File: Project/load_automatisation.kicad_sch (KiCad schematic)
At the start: 32 parts, among them IC1 TD62083AFGNEL, IC10 TD62083AFGNEL, IC2 TD62083AFGNEL, IC3 MC74VHC138DR2G, IC4 MC74VHC138DR2G, IC5 MC74VHC138DR2G, IC6 TD62083AFGNEL, IC7 TD62083AFGNEL, IC8 TD62083AFGNEL, IC9 LM358PWG4, J10 TENGConnector, J11 TENG, J12 PH-2X05SG, J19 DaqConnector, J9 PowerIn, Q1 2N5457, Q2 2N5457, U1 AMS1117-5.0, U2 INA128

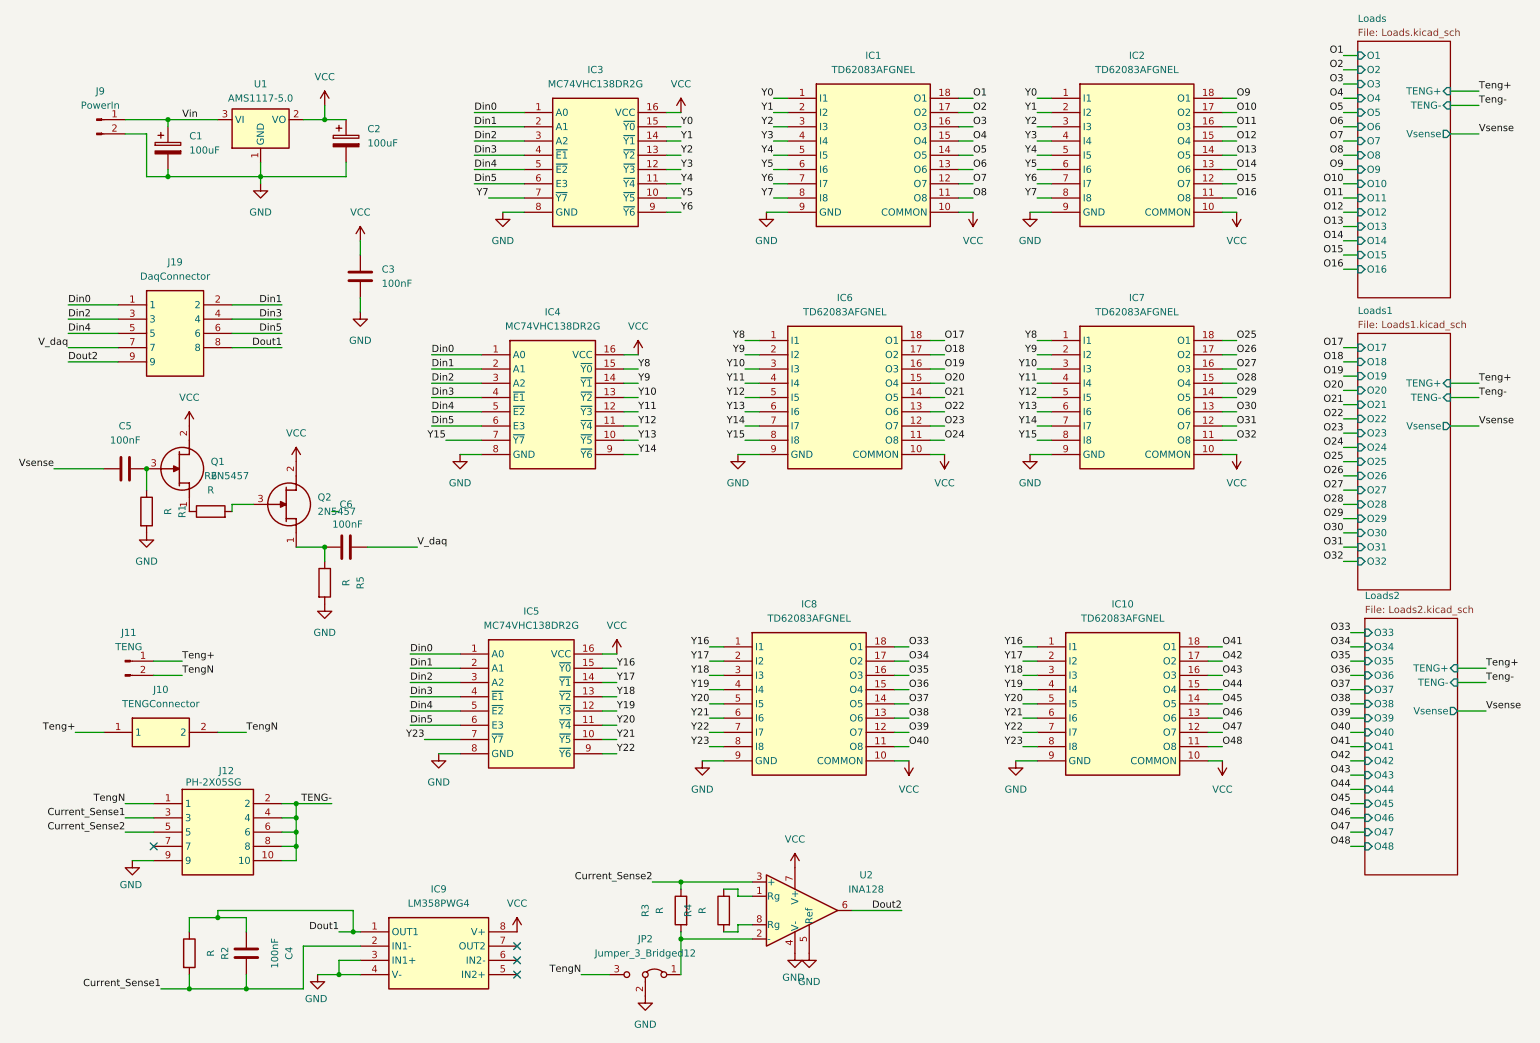
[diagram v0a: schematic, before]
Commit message: new 08/11
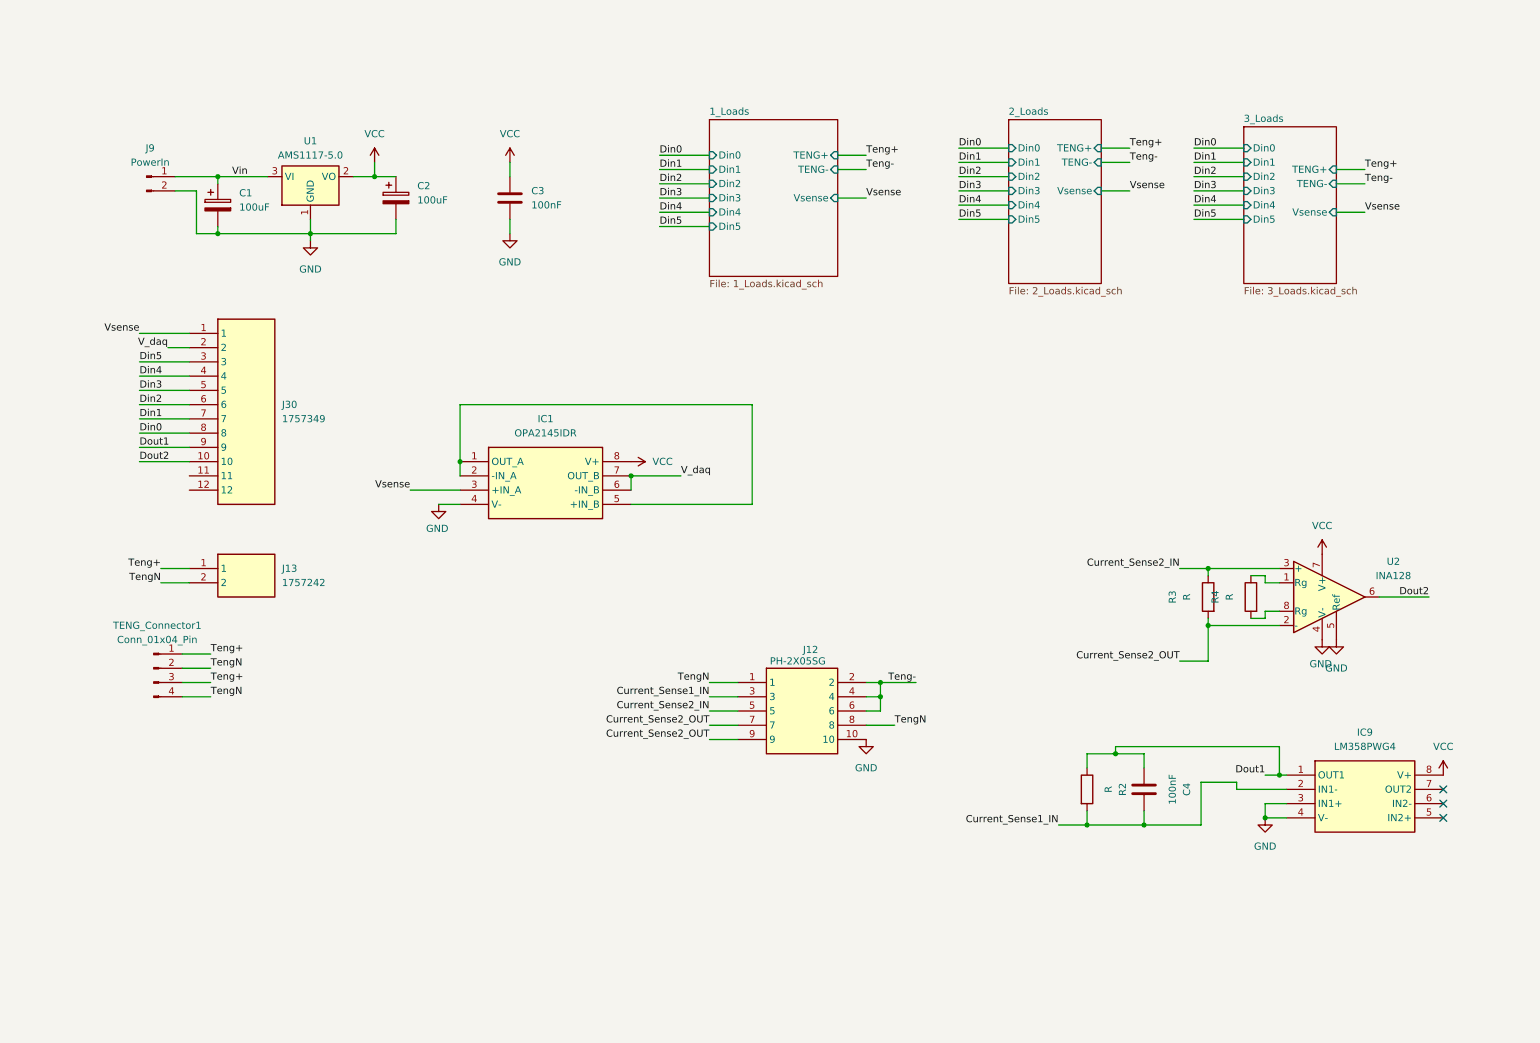
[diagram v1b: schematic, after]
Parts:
- removed C5, C6: 100nF, Capacitor_SMD:C_0805_2012Metric, symbol Device:C
- removed IC1, IC10, IC2, IC6, IC7, IC8: TD62083AFGNEL, SOIC127P1030X245-18N, symbol SamacSys_Parts:TD62083AFGNEL
- removed IC3: MC74VHC138DR2G, Library:SOIC127P600X175-16N, symbol SamacSys_Parts:MC74VHC138DR2G
- removed IC4, IC5: MC74VHC138DR2G, SamacSys_Parts:SOIC127P600X175-16N, symbol SamacSys_Parts:MC74VHC138DR2G
- removed J10: TENGConnector, 231162001000, symbol SamacSys_Parts:231-162_001-000
- removed J11: TENG, Connector_PinHeader_2.54mm:PinHeader_1x02_P2.54mm_Vertical, symbol Connector:Conn_01x02_Pin
- removed J19: DaqConnector, 231339001000, symbol SamacSys_Parts:231-339_001-000
- removed JP2: Jumper_3_Bridged12, Jumper:SolderJumper-3_P1.3mm_Bridged2Bar12_Pad1.0x1.5mm_NumberLabels, symbol Jumper:Jumper_3_Bridged12
- removed Q1, Q2: 2N5457, PN4117, symbol SamacSys_Parts:2N5457
- removed R1, R5, R6: R, Resistor_SMD:R_0805_2012Metric, symbol Device:R
- added IC1: OPA2145IDR, SOIC127P600X175-8N, symbol SamacSys_Parts:OPA2145IDR
- added J13: 1757242, 1757242, symbol SamacSys_Parts:1757242
- added J30: 1757349, SHDRRA12W103P0X508_1X12_6296X1200X875P, symbol SamacSys_Parts:1757349
- added TENG_Connector1: Conn_01x04_Pin, Connector_PinHeader_2.54mm:PinHeader_1x04_P2.54mm_Vertical, symbol Connector:Conn_01x04_Pin
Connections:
- net Din0: now also J30.8
- net Din1: now also J30.7
- net Din2: now also J30.6
- net Din3: now also J30.5
- net Din4: now also J30.4
- net Din5: now also J30.3
- net Dout1: now also J30.9
- net Dout2: now also J30.10
- net GND: now also J12.10, IC1.4 (V-); no longer J12.9
- net Teng+: now also J13.1, TENG_Connector1.1 (Pin_1), TENG_Connector1.3 (Pin_3)
- net Teng-: now also J12.2, J12.4, J12.6
- net TengN: now also J12.8, J13.2, TENG_Connector1.2 (Pin_2), TENG_Connector1.4 (Pin_4)
- net VCC: now also IC1.8 (V+)
- net V_daq: now also IC1.6 (-IN_B), IC1.7 (OUT_B), J30.2
- net Vsense: now also IC1.3 (+IN_A), J30.1
- net Current_Sense2_OUT: now reaches J12.7
- net Current_Sense2_OUT: now also J12.9, R3.2, U2.2 (-)
- net Current_Sense1 renamed Current_Sense1_IN
- net Current_Sense2 renamed Current_Sense2_IN
- removed net TENG-: J12.10, J12.2, J12.4, J12.6, J12.8
- new net: IC1.1 (OUT_A), IC1.2 (-IN_A), IC1.5 (+IN_B)
- no-connect marks 4 -> 3
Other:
- removed sheet Loads
- removed sheet Loads1
- removed sheet Loads2
- added sheet 1_Loads (1_Loads.kicad_sch)
- added sheet 2_Loads (2_Loads.kicad_sch)
- added sheet 3_Loads (3_Loads.kicad_sch)
- moved on the sheet: C1, C2, C3, C4, IC9, J12, J9, R2, R3, R4, U1, U2
